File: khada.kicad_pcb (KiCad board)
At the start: 2 copper layers, 154.2 x 111.4 mm, 56 parts, among them J1 MJ-4PP-9, SW1 SW_Push, SW10 SW_Push, SW11 SW_Push, SW12 SW_Push, SW13 SW_Push, SW14 SW_Push, SW15 SW_Push, SW16 SW_Push, SW17 SW_Push, SW18 SW_Push, SW19 SW_Push, SW2 SW_Push, SW20 SW_Push, SW21 SW_Push, SW22 SW_Push, SW3 SW_Push, SW4 SW_Push, SW5 SW_Push, SW6 SW_Push, SW7 SW_Push, SW8 SW_Push, SW9 SW_Push, U1 YAAJ_WeAct_BlackPill_Part_Lik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

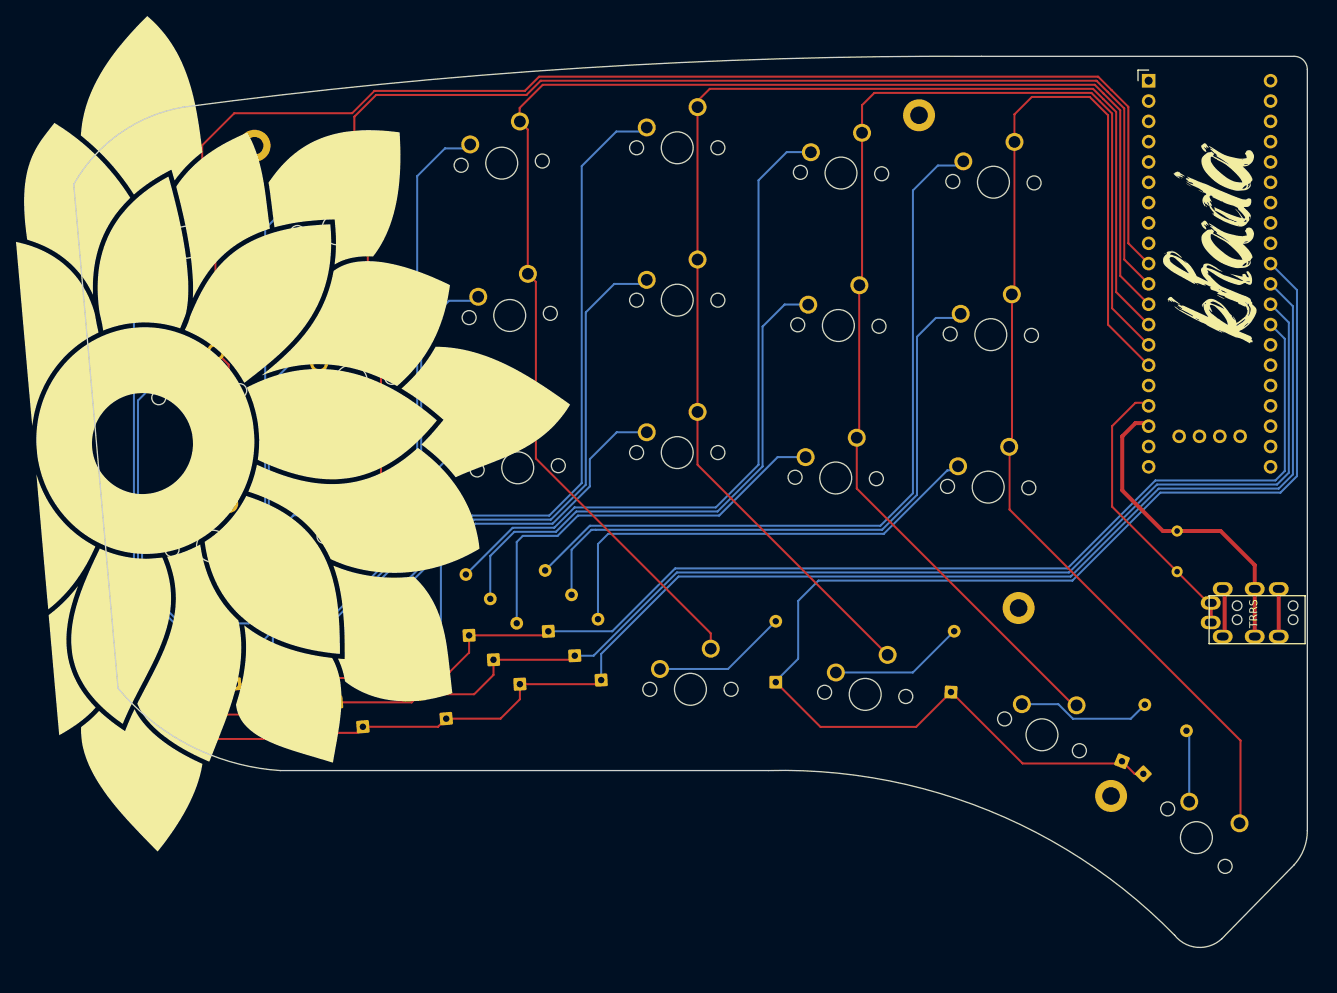
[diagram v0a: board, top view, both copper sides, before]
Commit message: final design unless wiring incorrect
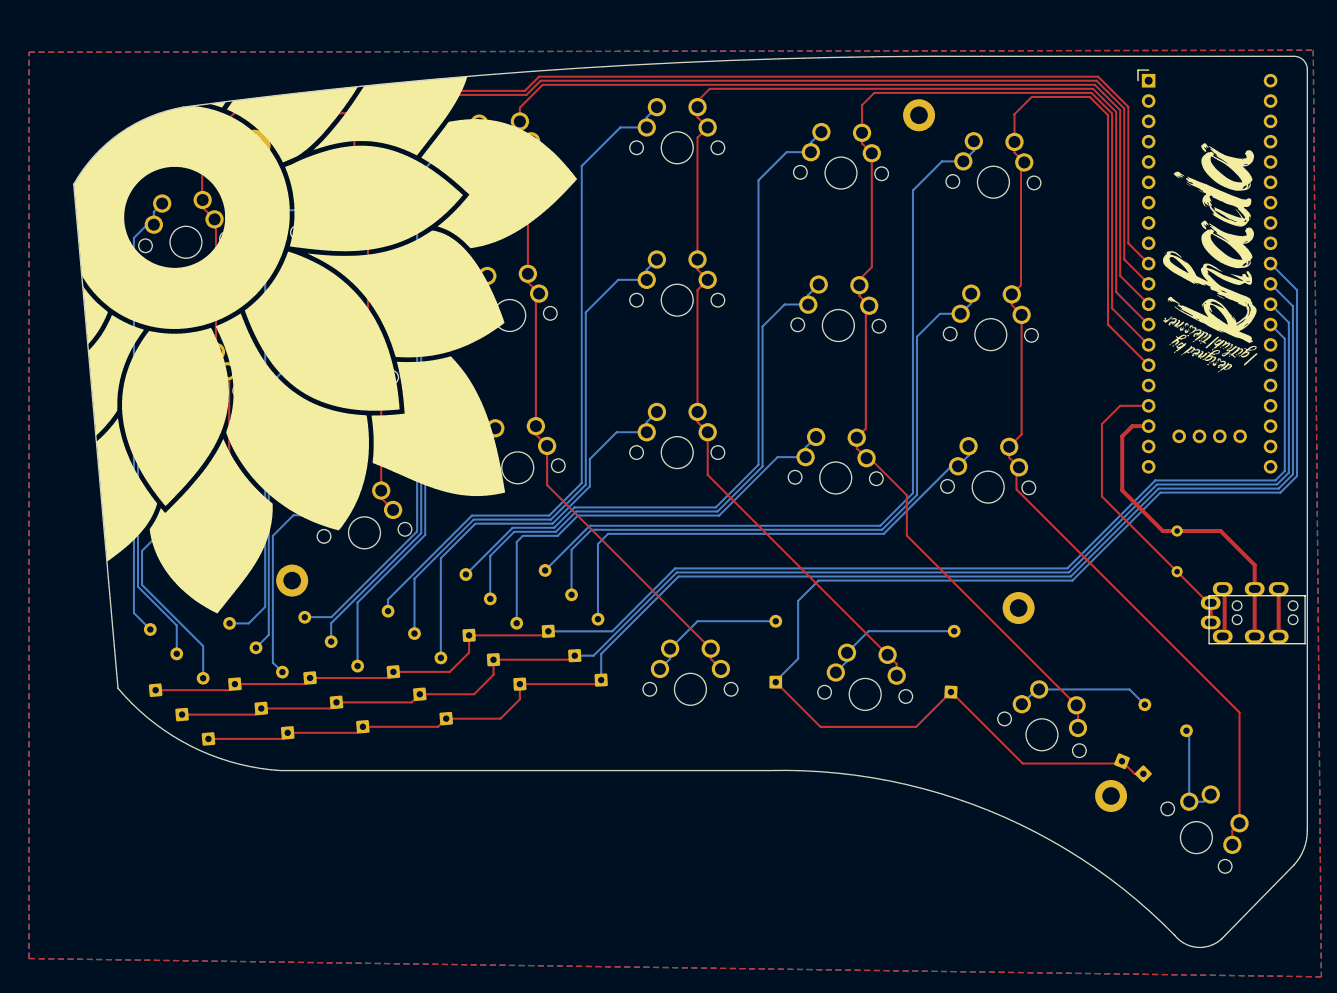
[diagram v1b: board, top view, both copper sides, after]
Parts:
- removed the G*** at (76.5, 94.9) (x2)
- added G***: LOGO, logo:designRed, F.Cu at (192.4, 85.2)
- added G***: LOGO, logo:lotusFront, F.Cu at (82.3, 85.1)
- added G***: LOGO, logo:lotusBack, B.Cu at (81.9, 85.3)
- added G***: LOGO, logo:designRed, B.Cu at (193.2, 85.2)
- SW1, SW10, SW12, SW13, SW14, SW15, SW16, SW17, SW18, SW19, SW2, SW20, SW21, SW22, SW3, SW4, SW5: footprint MX_Only:MXOnly-1U-NoLED -> switches:SW_MX_reversible_NoSilk
- SW11, SW6, SW7, SW8, SW9: footprint mx_only:MXOnly-1U-NoLED -> switches:SW_MX_reversible_NoSilk
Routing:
- net col5: track 147.8 -> 153.9 mm
- net col3: track 161.5 -> 166.7 mm
- net col4: track 150.7 -> 155.6 mm
- net Net-(D2-Pad2): track 38.5 -> 42.2 mm
- net col2: track 180.8 -> 184.5 mm
- net Net-(D19-Pad2): track 95.4 -> 98.7 mm
- net Net-(D20-Pad2): track 77.9 -> 81.1 mm
- net Net-(D21-Pad2): track 58.3 -> 61.5 mm
- net Net-(D6-Pad2): track 26.0 -> 29.1 mm
- net Net-(D5-Pad2): track 40.9 -> 44.0 mm
- net Net-(D4-Pad2): track 58.6 -> 61.7 mm
- net Net-(D22-Pad2): track 9.86 -> 12.9 mm
- net Net-(D13-Pad2): track 46.7 -> 49.8 mm
- net Net-(D16-Pad2): track 68.4 -> 71.4 mm
- net Net-(D17-Pad2): track 50.7 -> 53.7 mm
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- added copper zone on B.Cu, net GND
- added copper zone on F.Cu, net GND
